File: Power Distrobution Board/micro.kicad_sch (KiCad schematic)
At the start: 8 parts, among them CN2 NUCLEO-L432KC, U13 CD74HC4067M, U18 ISO1050DUB

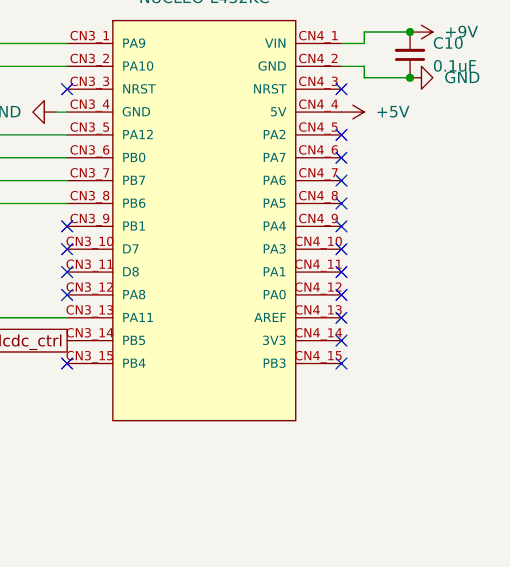
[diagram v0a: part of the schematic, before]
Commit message: commit 1 of v2
pd board v2 work first commit
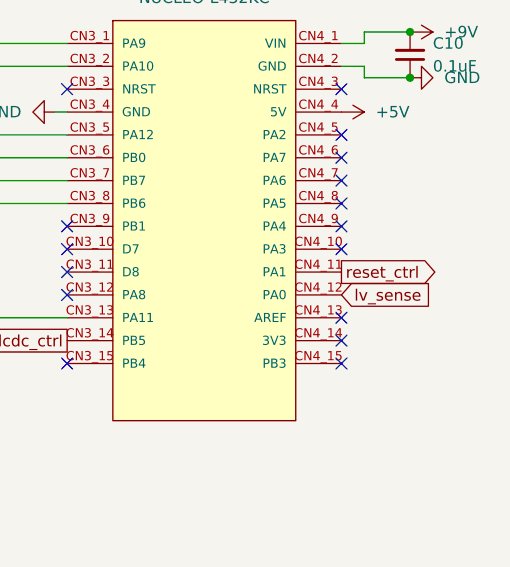
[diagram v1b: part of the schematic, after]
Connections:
- net reset_ctrl: now reaches CN2.CN4_11 (PA1)
- net lv_sense: now reaches CN2.CN4_12 (PA0)
- no-connect marks 22 -> 20
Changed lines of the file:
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@@
-	)
-	(no_connect
-		(at 128.27 86.36)
 	)
 	(no_connect
@@
 	)
 	(no_connect
-		(at 128.27 83.82)
-	)
-	(no_connect
 		(at 97.79 83.82)
 	)
@@
 		)
 	)
+	(global_label "lv_sense"
+		(shape input)
+		(at 128.27 86.36 0)
+		(fields_autoplaced yes)
+		(effects
+			(font
+				(size 1.27 1.27)
+			)
+			(justify left)
+		)
+		(property "Intersheetrefs" "${INTERSHEET_REFS}"
+			(at 139.238 86.36 0)
+			(effects
+				(font
+					(size 1.27 1.27)
+				)
+				(justify left)
+				(hide yes)
+			)
+		)
+	)
 	(global_label "ready_to_move_viout"
 		(shape input)
@@
 				(hide yes)
 			)
+		)
+	)
+	(global_label "reset_ctrl"
+		(shape output)
+		(at 128.27 83.82 0)
+		(fields_autoplaced yes)
+		(effects
+			(font
+				(size 1.27 1.27)
+			)
+			(justify left)
+		)
+		(property "Intersheetrefs" "${INTERSHEET_REFS}"
+			(at 140.2057 83.82 0)
+			(effects
+				(font
+					(size 1.27 1.27)
+				)
+				(justify left)
+				(hide yes)
+			)
